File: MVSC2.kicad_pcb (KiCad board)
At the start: 4 copper layers, 88.1 x 95.6 mm, 340 parts, among them J1 USB_C-SIGNAL, J10 PWM3_OUT, J11 PWM_IN, J12 EXP-1, J13 Exp2-smd, J14 EXP-3, J15 EXP-2, J16 ADC0, J17 ESTP0, J18 ESTP1, J19 ESTP2, J2 SERV2, J20 ESTP3, J21 ESTP4, J22 ESTP5, J23 POWER, J24 CaEx2, J25 SERV0, J26 SERV1, J27 CaEx2, J28 CaEx3, J29 ADC1, J3 EXP0, J30 HSES, J31 HSES, J32 HSES, J33 CaEx3, J34 SERV3, J35 SERV4, J36 SERV5, J37 EXP-SERVO, J38 I2C, J39 UART_pin, J4 EXP1, J40 UART, J41 I2C_pin, J42 I2C, J5 UART, J6 PWM0_OUT, J7 PWM1_OUT, J8 Exp1-pin, J9 PWM2_OUT, P1 STP0, P2 STP2, P3 STP4, P4 STP1, P5 STP3, P6 STP5, P7 CaEx4, P8 CaEx4, Q1 AO3400A, Q10 AO3400A, Q2 AO3400A, Q3 AO3400A, Q4 AO3400A, Q5 AO3400A, Q6 AO3400A, SW1 SKRKAEE020, SW2 SKRKAEE020, U1 XC6206P332MR, U10 TMC2208-LA-T, U11 TMC2208-LA-T, U12 TMC2208-LA-T, U3 STM32F411RCT6, U4 CH912LSR, U5 TMC2208-LA-T, U6 TMC2208-LA-T, U7 TMC2208-LA-T, U8 CH912LSR, U9 CH912LSR, Y1 25MHZ 12pF, Y2 32.768KHz 12.5pF

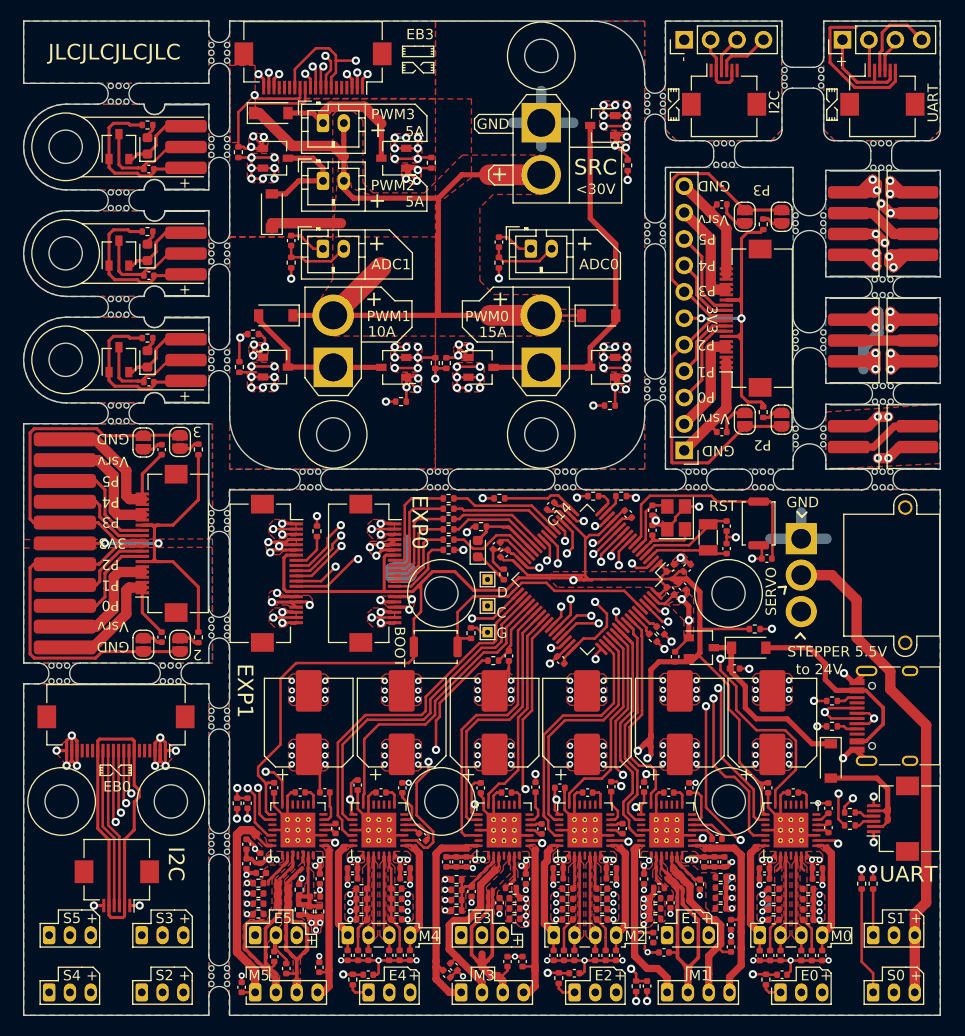
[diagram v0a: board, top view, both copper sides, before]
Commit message: working
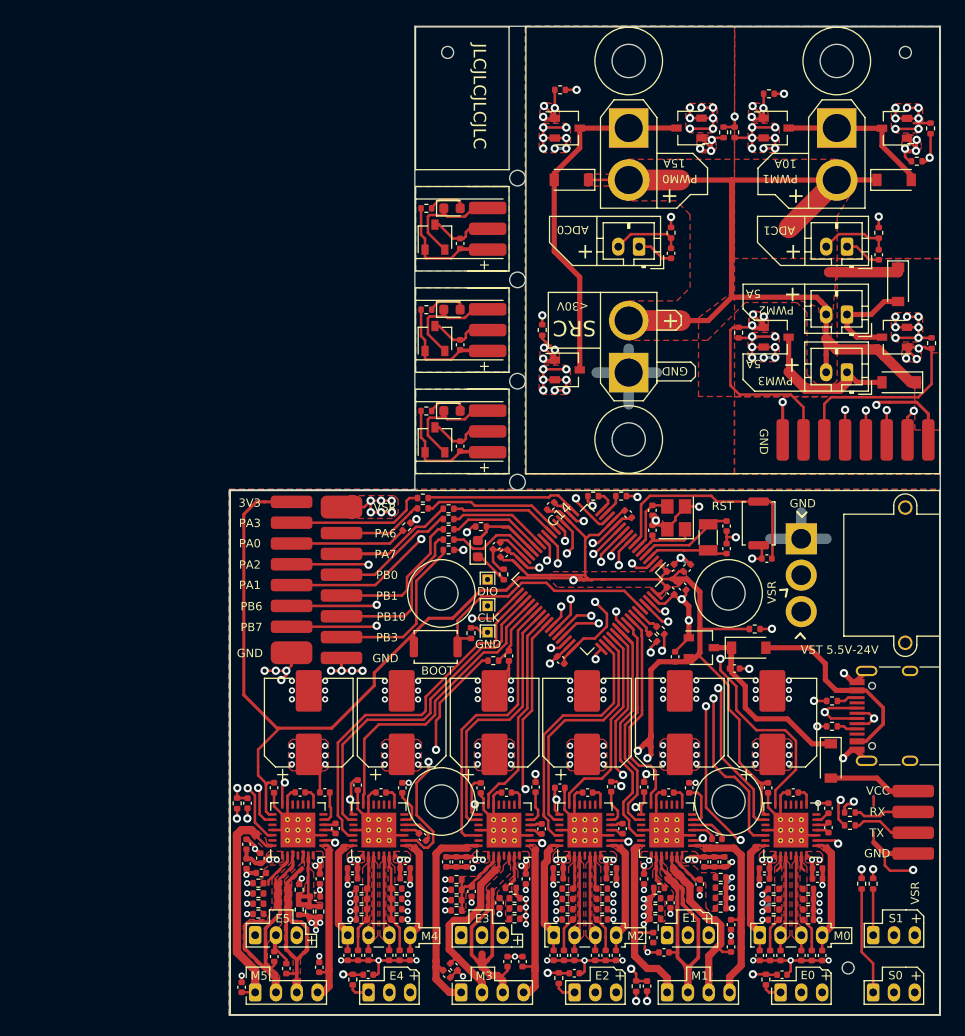
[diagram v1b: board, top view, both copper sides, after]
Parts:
- removed C120, C121, C2, C4: 4.7uF 10V, Capacitor_SMD:C_0402_1005Metric
- removed J12: EXP-1, Connector_FFC-FPC:Hirose_FH12-20S-0.5SH_1x20-1MP_P0.50mm_Horizontal
- removed J13: Exp2-smd, Connector_PinHeader_2.00mm:PinHeader_1x11_P2.00mm_Horizontal
- removed J14: EXP-3, Connector_FFC-FPC:Hirose_FH12-20S-0.5SH_1x20-1MP_P0.50mm_Horizontal
- removed J15: EXP-2, Connector_FFC-FPC:Hirose_FH12-20S-0.5SH_1x20-1MP_P0.50mm_Horizontal
- removed J24, J27: CaEx2, Connector_JST:JST_PH_B2B-PH-K_1x02_P2.00mm_Vertical
- removed J28, J33: CaEx3, Connector_JST:JST_PH_B3B-PH-K_1x03_P2.00mm_Vertical
- removed J34: SERV3, Connector_JST:JST_PH_B3B-PH-K_1x03_P2.00mm_Vertical
- removed J35: SERV4, Connector_JST:JST_PH_B3B-PH-K_1x03_P2.00mm_Vertical
- removed J36: SERV5, Connector_JST:JST_PH_B3B-PH-K_1x03_P2.00mm_Vertical
- removed J37: EXP-SERVO, Connector_FFC-FPC:Hirose_FH12-20S-0.5SH_1x20-1MP_P0.50mm_Horizontal
- removed J38, J42: I2C, Connector_FFC-FPC:Hirose_FH12-6S-0.5SH_1x06-1MP_P0.50mm_Horizontal
- removed J39: UART_pin, Connector_PinHeader_2.54mm:PinHeader_1x04_P2.54mm_Vertical
- removed J40, J5: UART, Connector_FFC-FPC:Hirose_FH12-6S-0.5SH_1x06-1MP_P0.50mm_Horizontal
- removed J41: I2C_pin, Connector_PinHeader_2.54mm:PinHeader_1x04_P2.54mm_Vertical
- removed J8: Exp1-pin, Connector_PinHeader_2.54mm:PinHeader_1x11_P2.54mm_Vertical
- removed JP1, JP2, JP3, JP4, JP5, JP6, JP7, JP8: SJ_O, Jumper:SolderJumper-2_P1.3mm_Open_RoundedPad1.0x1.5mm
- removed P7, P8: CaEx4, Connector_JST:JST_PH_B4B-PH-K_1x04_P2.00mm_Vertical
- removed R13, R14, R15, R16: 4.7k, Resistor_SMD:R_0402_1005Metric
- removed mouse-bite-2mm-slot (x32): VAL**, Panelization:mouse-bite-2mm-slot
- added P9: UART, Connector_JST:JST_PH_B4B-PH-K_1x04_P2.00mm_Vertical, F.Cu at (182.8, 155.0)
- added REF**: ToolingHole, MountingHole:MountingHole_3.2mm_M3, F.Cu at (178.0, 78.0)
- added REF**: MountingHole_3.2mm_M3, MountingHole:MountingHole_3.2mm_M3, F.Cu at (165.0, 130.0)
- added REF**: MountingHole_3.2mm_M3, MountingHole:MountingHole_3.2mm_M3, F.Cu at (137.4, 130.0)
- added REF**: MountingHole_3.2mm_M3, MountingHole:MountingHole_3.2mm_M3, F.Cu at (165.0, 150.0)
- added REF**: MountingHole_3.2mm_M3, MountingHole:MountingHole_3.2mm_M3, F.Cu at (137.4, 150.0)
- added REF**: MountingHole_3.2mm_M3, MountingHole:MountingHole_3.2mm_M3, F.Cu at (155.4, 115.2)
- added REF**: MountingHole_3.2mm_M3, MountingHole:MountingHole_3.2mm_M3, F.Cu at (175.4, 78.8)
- added REF**: MountingHole_3.2mm_M3, MountingHole:MountingHole_3.2mm_M3, F.Cu at (155.4, 78.8)
- added REF**: ToolingHole, MountingHole:MountingHole_3.2mm_M3, F.Cu at (180.0, 78.0)
- added REF**: ToolingHole, MountingHole:MountingHole_3.2mm_M3, F.Cu at (176.6, 166.0)
- added REF**: MountingHole_3.2mm_M3, MountingHole:MountingHole_3.2mm_M3, F.Cu at (144.7, 119.3)
- added REF**: MountingHole_3.2mm_M3, MountingHole:MountingHole_3.2mm_M3, F.Cu at (144.7, 109.6)
- added REF**: MountingHole_3.2mm_M3, MountingHole:MountingHole_3.2mm_M3, F.Cu at (144.7, 99.8)
- added REF**: MountingHole_3.2mm_M3, MountingHole:MountingHole_3.2mm_M3, F.Cu at (144.7, 90.0)
- J2: value SERV2 -> EXP0; footprint Connector_JST:JST_PH_B3B-PH-K_1x03_P2.00mm_Vertical -> Connector_PinHeader_2.00mm:PinHeader_1x08_P2.00mm_Vertical; moved to F.Cu
- J3: value EXP0 -> EXP1; footprint Connector_FFC-FPC:Hirose_FH12-20S-0.5SH_1x20-1MP_P0.50mm_Horizontal -> Connector_PinHeader_2.00mm:PinHeader_1x08_P2.00mm_Vertical
- J4: value EXP1 -> EXPB; footprint Connector_FFC-FPC:Hirose_FH12-20S-0.5SH_1x20-1MP_P0.50mm_Horizontal -> Connector_PinHeader_2.00mm:PinHeader_1x08_P2.00mm_Vertical
- moved R2 70.3 mm to (184.4, 85.3), turned to 90 degrees
- moved R26 69.1 mm to (184.5, 105.9), turned to 90 degrees
- moved R11 65.9 mm to (183.1, 88.5), turned to 180 degrees
- moved D6 65.7 mm to (181.4, 109.7), turned to 180 degrees
- moved Q3 63.8 mm to (181.0, 85.3), turned to 180 degrees
- moved Q10 61.9 mm to (181.0, 105.4), turned to 180 degrees
- moved D5 60.8 mm to (180.9, 90.3), turned to 0 degrees
- moved D9 60.6 mm to (181.3, 100.3), turned to 270 degrees
- moved R39 56.5 mm to (179.4, 95.3), turned to 90 degrees
- moved C26 56.5 mm to (179.4, 97.5), turned to 90 degrees
- moved J10 55.8 mm to (176.4, 108.7), turned to 180 degrees
- moved J7 53.6 mm to (175.4, 85.3), turned to 270 degrees
- moved J9 52.0 mm to (176.4, 103.2), turned to 180 degrees
- moved J29 50.4 mm to (176.4, 96.7), turned to 180 degrees
- moved J4 50.3 mm to (170.2, 115.2), turned to 90 degrees
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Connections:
- net GND_E3 renamed GND_EB
- net V_PWM_E3 renamed V_PWM_EB
- C25 pad 1: ADCGND_E3 -> GND_EB_ADC
- C26 pad 1: ADCGND_E3 -> GND_EB_ADC
- J16 pad 1: ADCGND_E3 -> GND_EB_ADC
- J2 pad 1: PWM0_E0 -> GND
- J2 pad 2: GND_E0 -> Net-(J2-Pad2)
- J2 pad 3: V_SERVO_E0 -> Net-(J2-Pad3)
- J29 pad 1: ADCGND_E3 -> GND_EB_ADC
- J3 pad 2: GND -> Net-(J3-Pad2)
- J3 pad 3: GND -> Net-(J3-Pad3)
- J3 pad 4: V_SERVO -> Net-(J3-Pad4)
- J3 pad 5: V_SERVO -> Net-(J3-Pad5)
- J3 pad 6: V_SERVO -> Net-(J3-Pad6)
- J3 pad 7: +3V3 -> Net-(J3-Pad7)
- J3 pad 8: Net-(J3-Pad8) -> V_SERVO
- J4 pad 1: GND -> GND_EB_ADC
- J4 pad 2: GND -> PWM3_E3
- J4 pad 3: GND -> PWM2_E3
- J4 pad 4: V_SERVO -> ADC1
- J4 pad 5: V_SERVO -> ADC0
- J4 pad 6: V_SERVO -> PWM1_E3
- J4 pad 7: +3V3 -> PWM0_E3
- J4 pad 8: Net-(J4-Pad8) -> 3V3_EB
- R31 pad 2: 3v3_E3 -> 3V3_EB
- R32 pad 2: Net-(J3-Pad8) -> Net-(J3-Pad7)
- R33 pad 2: Net-(J3-Pad9) -> Net-(J3-Pad6)
- R34 pad 2: Net-(J3-Pad10) -> Net-(J3-Pad5)
- R35 pad 2: Net-(J3-Pad11) -> Net-(J3-Pad4)
- R36 pad 2: Net-(J3-Pad12) -> Net-(J3-Pad3)
- R37 pad 2: Net-(J3-Pad13) -> Net-(J3-Pad2)
- R38 pad 2: Net-(J4-Pad9) -> Net-(J2-Pad7)
- R39 pad 2: 3v3_E3 -> 3V3_EB
- R40 pad 2: Net-(J4-Pad10) -> Net-(J2-Pad5)
- R41 pad 2: Net-(J4-Pad11) -> Net-(J2-Pad4)
- R42 pad 2: Net-(J4-Pad8) -> Net-(J2-Pad6)
- R43 pad 2: Net-(J4-Pad12) -> Net-(J2-Pad3)
- R44 pad 2: Net-(J4-Pad13) -> Net-(J2-Pad2)
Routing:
- net 3v3_E3: track 87.2 -> 0.00 mm, vias 3 -> 0
- net 3V3_EB: track 0.00 -> 75.7 mm, vias 0 -> 3
- net Net-(J2-Pad2): track 0.00 -> 53.1 mm, vias 0 -> 2
- net GND_EB_ADC: track 0.00 -> 51.1 mm, vias 0 -> 1
- net ADCGND_E3: track 51.6 -> 0.88 mm, vias 1 -> 0
- net Net-(J2-Pad3): track 0.00 -> 49.2 mm, vias 0 -> 2
- net Net-(J4-Pad13): track 46.9 -> 0.00 mm, vias 2 -> 0
- net Net-(J4-Pad12): track 45.8 -> 0.00 mm, vias 2 -> 0
- net 3v3_E0: track 40.1 -> 0.00 mm
- net Net-(J2-Pad4): track 0.00 -> 37.8 mm, vias 0 -> 2
- net Net-(J4-Pad11): track 37.7 -> 0.00 mm, vias 2 -> 0
- net Net-(J13-Pad6): track 36.7 -> 0.00 mm, vias 2 -> 0
- net Net-(J13-Pad7): track 35.8 -> 0.00 mm
- net Net-(J13-Pad5): track 35.8 -> 0.00 mm
- net Net-(J2-Pad5): track 0.00 -> 33.6 mm, vias 0 -> 2
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- added copper zone on F.Cu, net GND_EB_ADC
- removed copper zone on F.Cu, net (none)
- removed copper zone on B.Cu, net GND_E0
- removed copper zone on F.Cu, net GND_E0
- removed copper zone on In1.Cu, net GND_E0
- removed copper zone on In2.Cu, net GND_E0
- removed copper zone on F.Cu, net Net-(C120-Pad1)
- removed copper zone on F.Cu, net Net-(C121-Pad1)
- removed copper zone on F.Cu, net Net-(C27-Pad2)
- removed copper zone on F.Cu, net Net-(C52-Pad2)
- removed copper zone on F.Cu, net Net-(C68-Pad2)
- removed copper zone on F.Cu, net Net-(D3-Pad2)
- removed copper zone on F.Cu, net Net-(J24-Pad1)
- removed copper zone on B.Cu, net Net-(J24-Pad2)
- removed copper zone on In1.Cu, net Net-(J24-Pad2)
- removed copper zone on In2.Cu, net Net-(J24-Pad2)
- removed copper zone on In2.Cu, net Net-(J28-Pad1)
- removed copper zone on B.Cu, net Net-(J28-Pad3)
- removed copper zone on In1.Cu, net Net-(J28-Pad3)
- removed copper zone on B.Cu, net Net-(J39-Pad2)
- removed copper zone on F.Cu, net Net-(J39-Pad2)
- removed copper zone on In1.Cu, net Net-(J39-Pad2)
- removed copper zone on In2.Cu, net Net-(J39-Pad2)
- removed copper zone on B.Cu, net Net-(J41-Pad1)
- removed copper zone on F.Cu, net Net-(J41-Pad1)
- removed copper zone on In1.Cu, net Net-(J41-Pad1)
- removed copper zone on In2.Cu, net Net-(J41-Pad1)
- removed copper zone on In1.Cu, net Net-(P7-Pad1)
- removed copper zone on B.Cu, net Net-(P7-Pad2)
- removed copper zone on In2.Cu, net Net-(P7-Pad4)
- removed copper zone on F.Cu, net V_SERVO_E0
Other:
- board size 88.1 x 95.6 mm -> 68.3 x 95.1 mm
- board text added: "PA0"
- board text added: "PA1"
- board text added: "PA2"
- board text added: "PA3"
- board text added: "PA6"
- board text added: "PA7"
- board text added: "PB0"
- board text added: "PB1"
- board text added: "PB10"
- board text added: "PB3"
- board text added: "PB6"
- board text added: "PB7"
- board text added: "RX"
- board text added: "TX"
- board text added: "VCC"
- board text added: "VSR"
- board text added: "VST 5.5V-24V"
- board text removed: "-"
- board text removed: "2"
- board text removed: "3"
- board text removed: "5V"
- board text removed: "A0 A3 A2"
- board text removed: "A0 A3 A2 A1 B6 B7"
- board text removed: "A1 B6 B7"
- board text removed: "A6 A7 B0 B1 B10 B3"
- board text removed: "A6 A7 B8 B1"
- board text removed: "B10"
- board text removed: "B3"
- board text removed: "EB0"
- board text removed: "EB1"
- board text removed: "EB2"
- board text removed: "EB3"
- board text removed: "EXP0"
- board text removed: "EXP1"
- board text removed: "I2C"
- board text removed: "P0"
- board text removed: "P0 P1 P2 P3 P4 P5"
- board text removed: "P1"
- board text removed: "P2"
- board text removed: "P3"
- board text removed: "P4"
- board text removed: "P5"
- board text removed: "P5 P4 P3 P2 P1 P0"
- board text removed: "RXD"
- board text removed: "S2"
- board text removed: "S3"
- board text removed: "S4"
- board text removed: "S5"
- board text removed: "SCL"
- board text removed: "SDA"
- board text removed: "SERVO"
- board text removed: "STEPPER 5.5V"
- board text removed: "TXD"
- board text removed: "UART"
- board text removed: "Vsrv"
- board text removed: "to 24V"
